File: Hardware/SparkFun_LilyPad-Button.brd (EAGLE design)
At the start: 15.7 x 8 mm, 6 parts

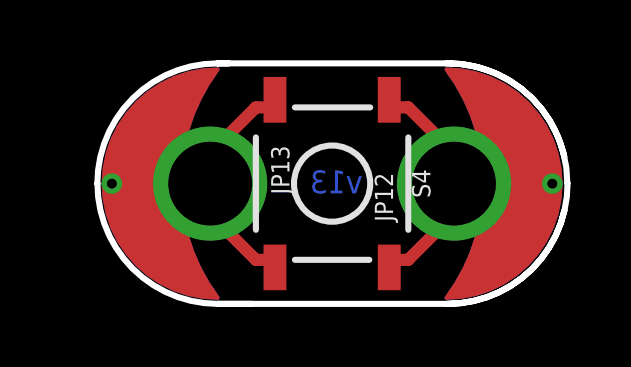
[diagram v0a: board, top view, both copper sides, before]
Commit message: Clean up a few things
Ready for review
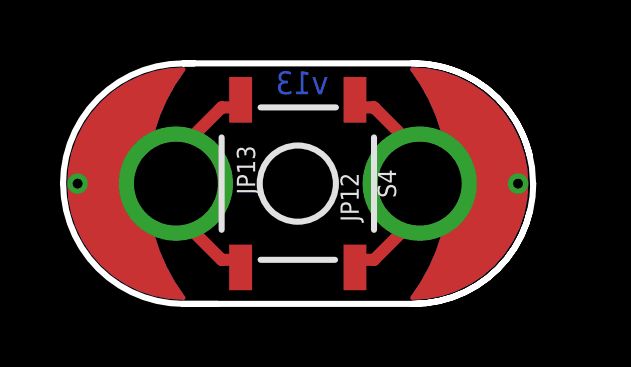
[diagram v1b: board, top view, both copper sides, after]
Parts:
- moved JP12 1.14 mm to (11.7, 4.01)
- moved JP13 1.14 mm to (4.06, 4.01)
- moved S4 1.14 mm to (7.87, 4.01)
- moved U$45 1.14 mm to (7.87, 4.01)
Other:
- board text added: "Inches"
- board text added: "Unplated holes: 0.013"
- board text removed: "Unplated holes: 0.02"
